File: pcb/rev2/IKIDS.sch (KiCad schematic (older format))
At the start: 41 parts, among them SW1 SW_Push, U1 ATmega32U4-AU, Y1 16MHz

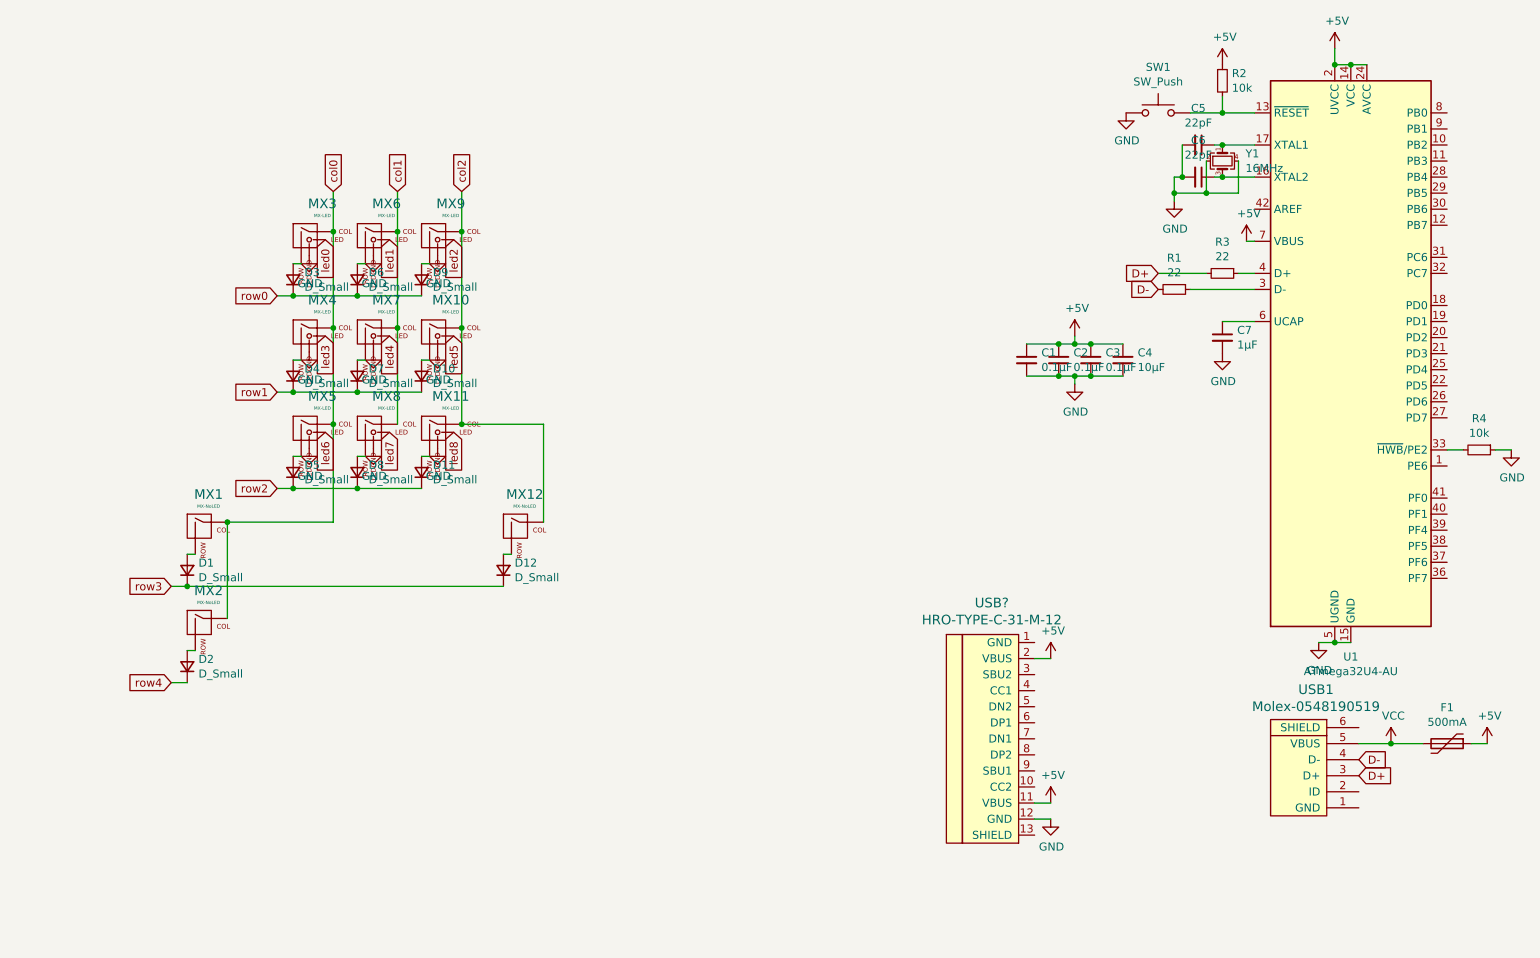
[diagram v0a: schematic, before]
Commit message: Added finished PCB to repo
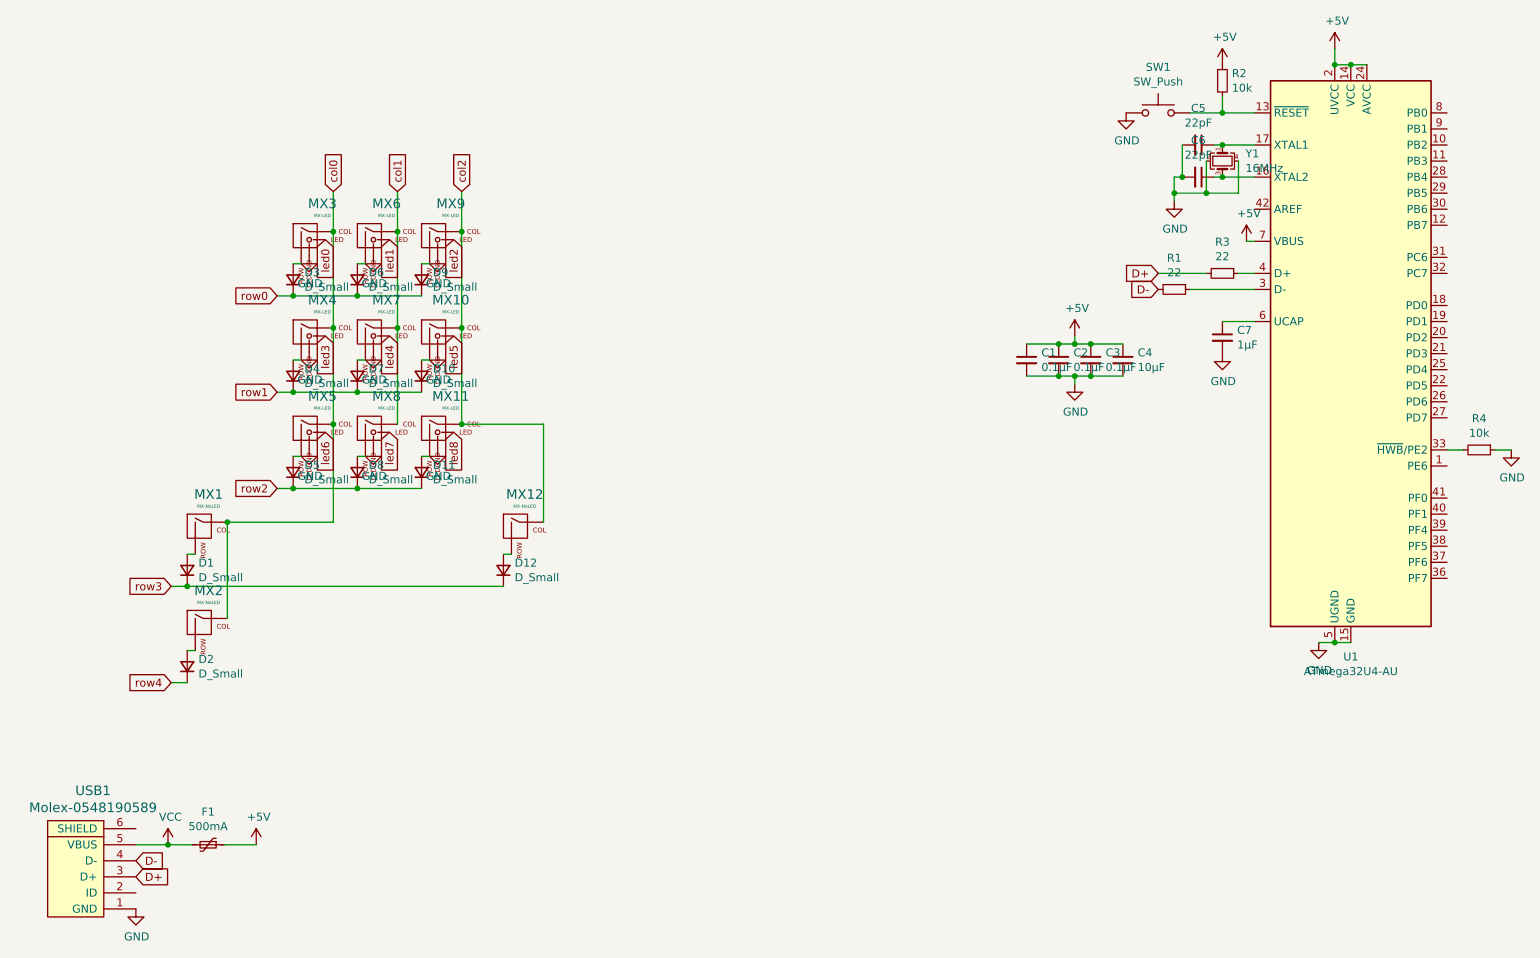
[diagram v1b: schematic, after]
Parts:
- removed F1: 500mA, Fuse:Fuse_1206_3216Metric, symbol Device:Polyfuse
- removed USB1: Molex-0548190519, random-keyboard-parts:Molex-0548190589, symbol random-keyboard-parts:Molex-0548190519
- removed USB?: HRO-TYPE-C-31-M-12, symbol keebio:HRO-TYPE-C-31-M-12
- added F1: 500mA, Fuse:Fuse_1206_3216Metric, symbol Device:Polyfuse_Small
- added USB1: Molex-0548190589, random-keyboard-parts:Molex-0548190589, symbol random-keyboard-parts:Molex-0548190589
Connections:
- net +5V: now also F1.1
- net D+: now also USB1.3 (D+)
- net D-: now also USB1.4 (D-)
- net GND: now also USB1.1 (GND)
- net VCC: now also F1.2, USB1.5 (VBUS)
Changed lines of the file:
@@
 Comment4 ""
 $EndDescr
-$Comp
-L MCU_Microchip_ATmega:ATmega32U4-AU U1
-U 1 1 607794AF
-P 9540 3080
-F 0 "U1" H 9540 1191 50  0000 C CNN
-F 1 "ATmega32U4-AU" H 9540 1100 50  0000 C CNN
-F 2 "Package_QFP:TQFP-44_10x10mm_P0.8mm" H 9540 3080 50  0001 C CIN
-F 3 "http://ww1.microchip.com/downloads/en/DeviceDoc/Atmel-7766-8-bit-AVR-ATmega16U4-32U4_Datasheet.pdf" H 9540 3080 50  0001 C CNN
-	1    9540 3080
-	1    0    0    -1
-$EndComp
-Wire Wire Line
-	9440 1280 9540 1280
-Connection ~ 9540 1280
-Wire Wire Line
-	9540 1280 9640 1280
 Wire Wire Line
 	9440 1280 9440 1180
-Connection ~ 9440 1280
 $Comp
 L power:+5V #PWR0101
@@
 	1    0    0    -1
 $EndComp
-Wire Wire Line
-	9540 4880 9440 4880
-Connection ~ 9440 4880
-Wire Wire Line
-	9440 4880 9340 4880
 $Comp
 L power:GND #PWR0102
@@
 	1    0    0    -1
 $EndComp
-$Comp
-L random-keyboard-parts:Molex-0548190519 USB1
-U 1 1 6077A7AA
-P 9290 5710
-F 0 "USB1" V 9827 5677 60  0000 C CNN
-F 1 "Molex-0548190519" V 9721 5677 60  0000 C CNN
-F 2 "random-keyboard-parts:Molex-0548190589" H 9290 5710 60  0001 C CNN
-F 3 "" H 9290 5710 60  0001 C CNN
-	1    9290 5710
-	0    -1   -1   0
-$EndComp
-Wire Wire Line
-	9590 5510 9790 5510
-$Comp
-L power:VCC #PWR0111
-U 1 1 6077D28D
-P 9790 5510
-F 0 "#PWR0111" H 9790 5360 50  0001 C CNN
-F 1 "VCC" H 9805 5683 50  0000 C CNN
-F 2 "" H 9790 5510 50  0001 C CNN
-F 3 "" H 9790 5510 50  0001 C CNN
-	1    9790 5510
-	1    0    0    -1
-$EndComp
-Wire Wire Line
-	9790 5510 9990 5510
-Connection ~ 9790 5510
-$Comp
-L Device:Polyfuse F1
-U 1 1 6077E43E
-P 10140 5510
-F 0 "F1" V 9915 5510 50  0000 C CNN
-F 1 "500mA" V 10006 5510 50  0000 C CNN
-F 2 "Fuse:Fuse_1206_3216Metric" H 10190 5310 50  0001 L CNN
-F 3 "~" H 10140 5510 50  0001 C CNN
-	1    10140 5510
-	0    1    1    0
-$EndComp
-Wire Wire Line
-	10290 5510 10390 5510
-$Comp
-L power:+5V #PWR0112
-U 1 1 6077F79A
-P 10390 5510
-F 0 "#PWR0112" H 10390 5360 50  0001 C CNN
-F 1 "+5V" H 10405 5683 50  0000 C CNN
-F 2 "" H 10390 5510 50  0001 C CNN
-F 3 "" H 10390 5510 50  0001 C CNN
-	1    10390 5510
-	1    0    0    -1
-$EndComp
-Text GLabel 9590 5610 2    50   Input ~ 0
-D-
-Text GLabel 9590 5710 2    50   Input ~ 0
-D+
 $Comp
 L MX_Alps_Hybrid:MX-LED MX3
@@
 Text GLabel 3950 3570 3    50   Input ~ 0
 led8
-$Comp
-L keebio:HRO-TYPE-C-31-M-12 USB?
-U 1 1 607E2252
-P 7470 5430
-F 0 "USB?" H 7303 6227 60  0000 C CNN
-F 1 "HRO-TYPE-C-31-M-12" H 7303 6121 60  0000 C CNN
-F 2 "" H 7470 5430 60  0001 C CNN
-F 3 "" H 7470 5430 60  0001 C CNN
-	1    7470 5430
-	1    0    0    -1
-$EndComp
-Wire Wire Line
-	7570 4980 7670 4980
-$Comp
-L power:+5V #PWR?
-U 1 1 607E72D0
-P 7670 4980
-F 0 "#PWR?" H 7670 4830 50  0001 C CNN
-F 1 "+5V" H 7685 5153 50  0000 C CNN
-F 2 "" H 7670 4980 50  0001 C CNN
-F 3 "" H 7670 4980 50  0001 C CNN
-	1    7670 4980
-	1    0    0    -1
-$EndComp
-Wire Wire Line
-	7570 5880 7670 5880
-$Comp
-L power:+5V #PWR?
-U 1 1 607EA54B
-P 7670 5880
-F 0 "#PWR?" H 7670 5730 50  0001 C CNN
-F 1 "+5V" H 7685 6053 50  0000 C CNN
-F 2 "" H 7670 5880 50  0001 C CNN
-F 3 "" H 7670 5880 50  0001 C CNN
-	1    7670 5880
-	1    0    0    -1
-$EndComp
-Wire Wire Line
-	7570 5980 7670 5980
-$Comp
-L power:GND #PWR?
-U 1 1 607EE216
-P 7670 5980
-F 0 "#PWR?" H 7670 5730 50  0001 C CNN
-F 1 "GND" H 7675 5807 50  0000 C CNN
-F 2 "" H 7670 5980 50  0001 C CNN
-F 3 "" H 7670 5980 50  0001 C CNN
-	1    7670 5980
-	1    0    0    -1
-$EndComp
+Connection ~ 9440 4880
+Wire Wire Line
+	9440 4880 9340 4880
+Wire Wire Line
+	9540 4880 9440 4880
+Connection ~ 9440 1280
+Connection ~ 9540 1280
+Wire Wire Line
+	9540 1280 9640 1280
+Wire Wire Line
+	9440 1280 9540 1280
+$Comp
+L MCU_Microchip_ATmega:ATmega32U4-AU U1
+U 1 1 607794AF
+P 9540 3080
+F 0 "U1" H 9540 1191 50  0000 C CNN
+F 1 "ATmega32U4-AU" H 9540 1100 50  0000 C CNN
+F 2 "Package_QFP:TQFP-44_10x10mm_P0.8mm" H 9540 3080 50  0001 C CIN
+F 3 "http://ww1.microchip.com/downloads/en/DeviceDoc/Atmel-7766-8-bit-AVR-ATmega16U4-32U4_Datasheet.pdf" H 9540 3080 50  0001 C CNN
+	1    9540 3080
+	1    0    0    -1
+$EndComp
+$Comp
+L random-keyboard-parts:Molex-0548190589 USB1
+U 1 1 6079F11B
+P 1670 6340
+F 0 "USB1" V 2207 6307 60  0000 C CNN
+F 1 "Molex-0548190589" V 2101 6307 60  0000 C CNN
+F 2 "random-keyboard-parts:Molex-0548190589" H 1670 6340 60  0001 C CNN
+F 3 "" H 1670 6340 60  0001 C CNN
+	1    1670 6340
+	0    -1   -1   0
+$EndComp
+Wire Wire Line
+	1970 6140 2170 6140
+$Comp
+L power:VCC #PWR0111
+U 1 1 607A247B
+P 2170 6140
+F 0 "#PWR0111" H 2170 5990 50  0001 C CNN
+F 1 "VCC" H 2185 6313 50  0000 C CNN
+F 2 "" H 2170 6140 50  0001 C CNN
+F 3 "" H 2170 6140 50  0001 C CNN
+	1    2170 6140
+	1    0    0    -1
+$EndComp
+Wire Wire Line
+	2170 6140 2320 6140
+Connection ~ 2170 6140
+$Comp
+L Device:Polyfuse_Small F1
+U 1 1 607A5C52
+P 2420 6140
+F 0 "F1" V 2215 6140 50  0000 C CNN
+F 1 "500mA" V 2306 6140 50  0000 C CNN
+F 2 "Fuse:Fuse_1206_3216Metric" H 2470 5940 50  0001 L CNN
+F 3 "~" H 2420 6140 50  0001 C CNN
+	1    2420 6140
+	0    1    1    0
+$EndComp
+Wire Wire Line
+	2520 6140 2720 6140
+$Comp
+L power:+5V #PWR0112
+U 1 1 607A8D6A
+P 2720 6140
+F 0 "#PWR0112" H 2720 5990 50  0001 C CNN
+F 1 "+5V" H 2735 6313 50  0000 C CNN
+F 2 "" H 2720 6140 50  0001 C CNN
+F 3 "" H 2720 6140 50  0001 C CNN
+	1    2720 6140
+	1    0    0    -1
+$EndComp
+$Comp
+L power:GND #PWR0122
+U 1 1 607A956C
+P 1970 6540
+F 0 "#PWR0122" H 1970 6290 50  0001 C CNN
+F 1 "GND" H 1975 6367 50  0000 C CNN
+F 2 "" H 1970 6540 50  0001 C CNN
+F 3 "" H 1970 6540 50  0001 C CNN
+	1    1970 6540
+	1    0    0    -1
+$EndComp
+Text GLabel 1970 6240 2    50   Input ~ 0
+D-
+Text GLabel 1970 6340 2    50   Input ~ 0
+D+
 $EndSCHEMATC
